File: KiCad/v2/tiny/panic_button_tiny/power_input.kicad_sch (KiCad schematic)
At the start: 8 parts, among them J2 Conn_USB_C_Socket_PowerOnly, U3 ME6211C33M5

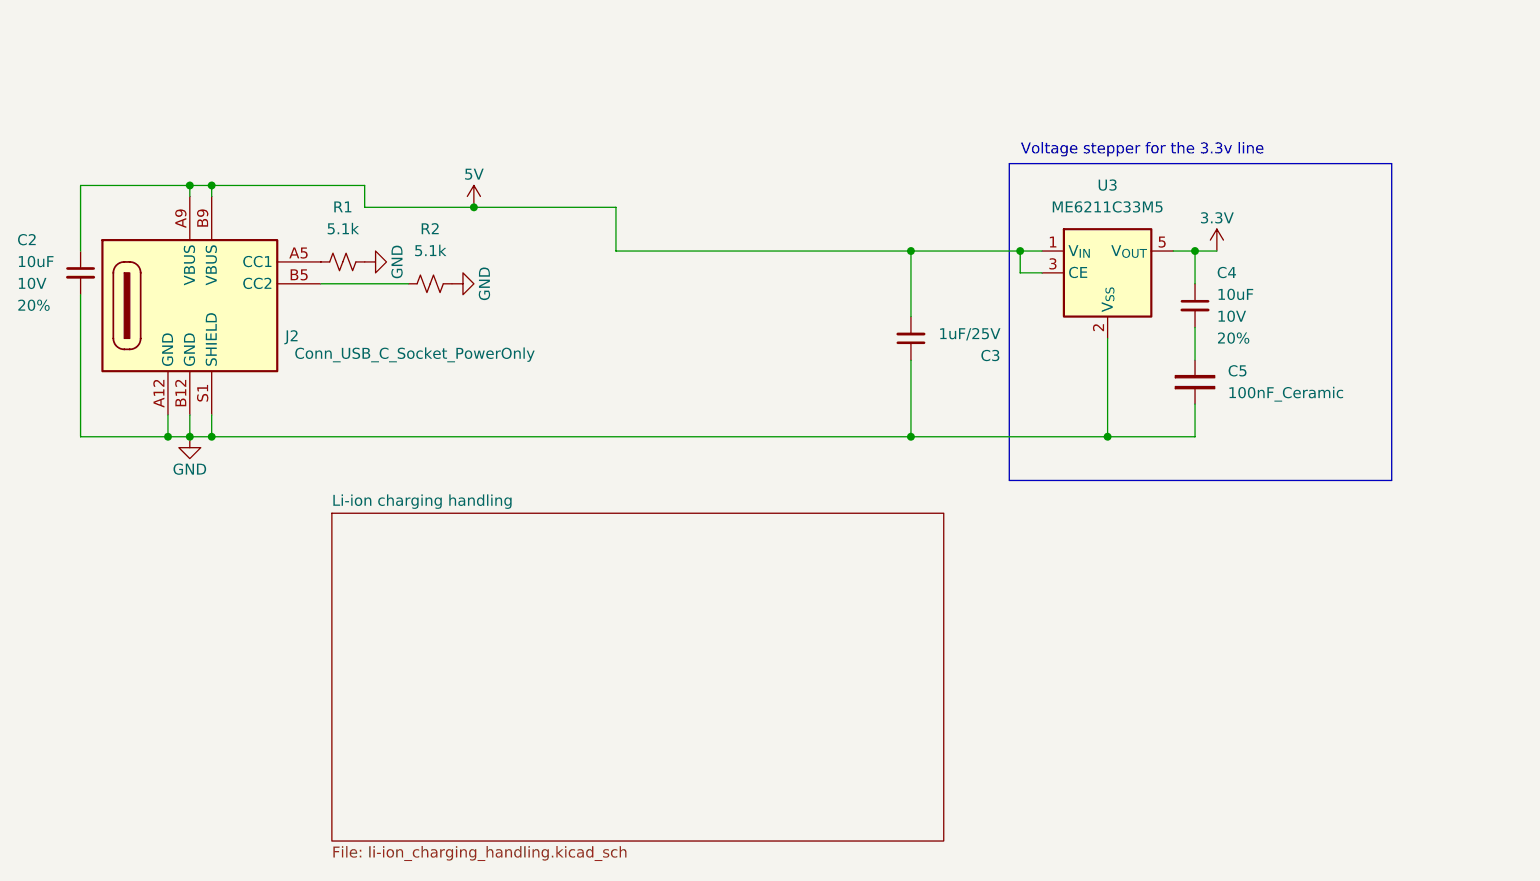
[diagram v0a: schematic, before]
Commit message: [UPDATE] the schematic wirering
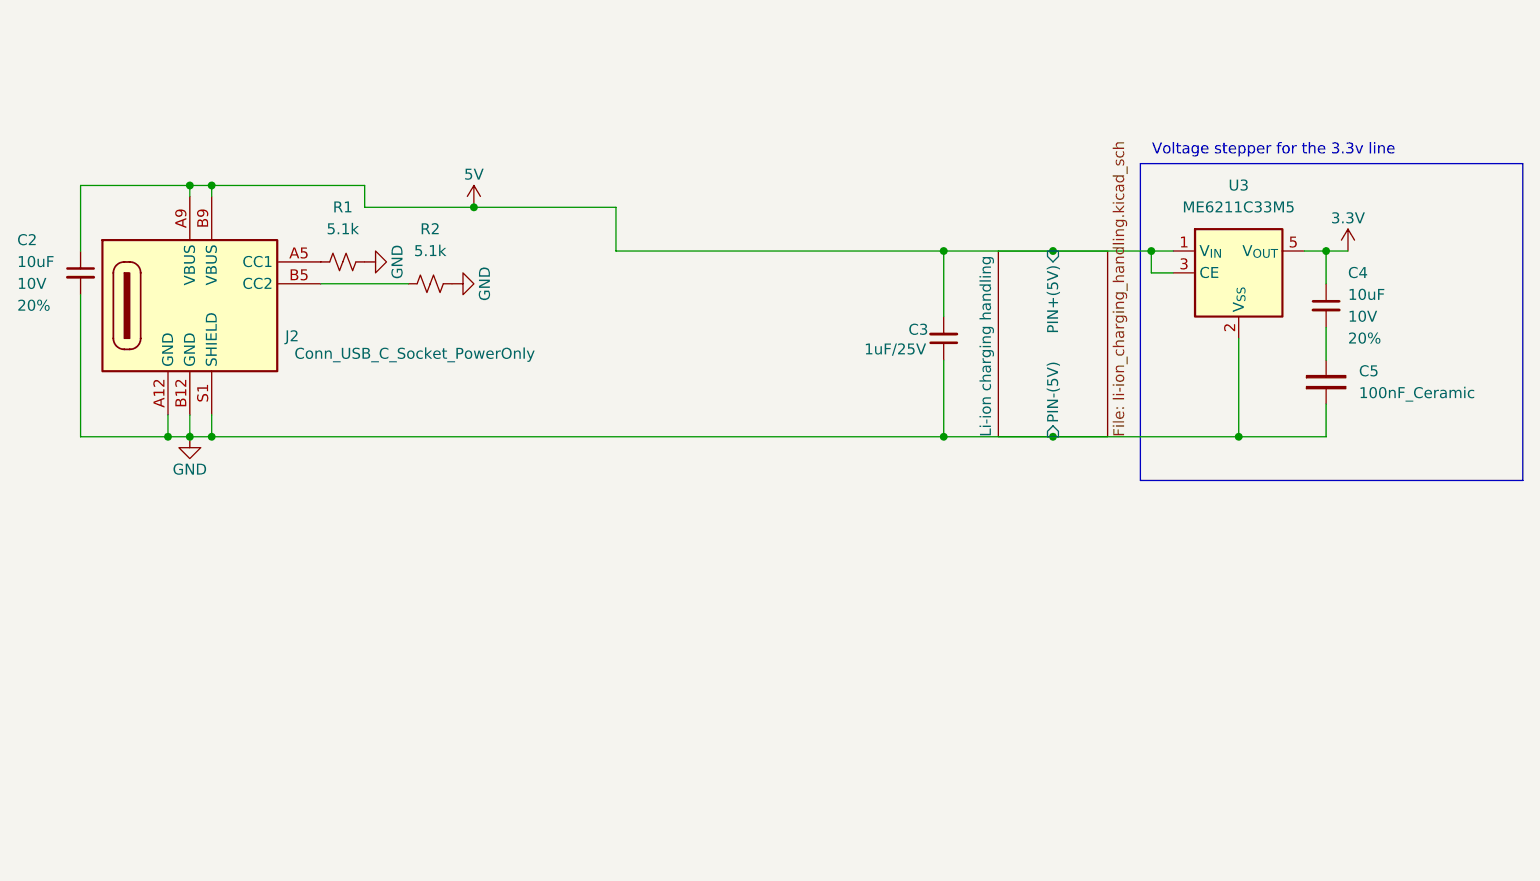
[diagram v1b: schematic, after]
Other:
- sheet Li-ion charging handling ports: added PIN+(5V), PIN-(5V); removed none
- moved on the sheet: C3, C4, C5, U3
